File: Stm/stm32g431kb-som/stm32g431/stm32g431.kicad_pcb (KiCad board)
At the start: 2 copper layers, 30 x 26.8 mm, 4 parts, among them J1 Conn_ARM_JTAG_SWD_10, U1 STM32G431KBTx, Y1 ECS-TXO-3225-250-TR

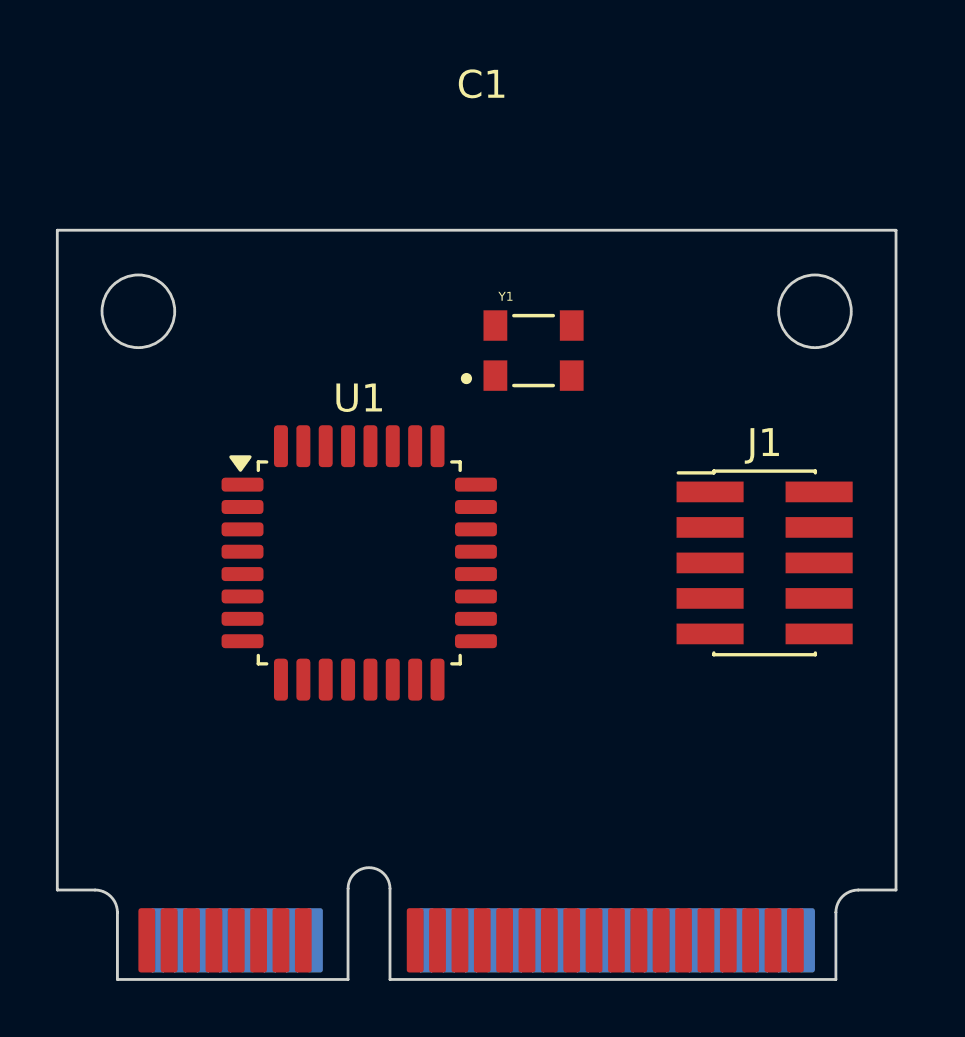
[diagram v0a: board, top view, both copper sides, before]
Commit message: Pcb
Add more components
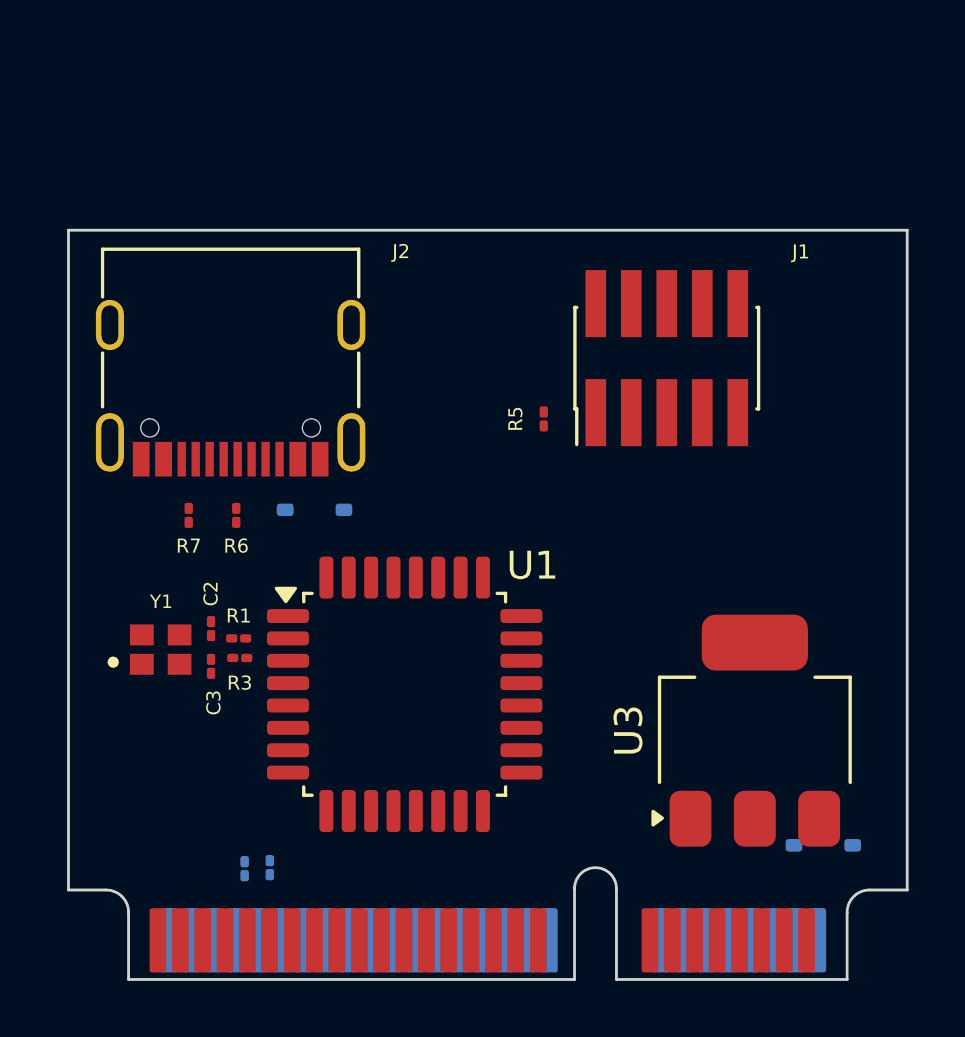
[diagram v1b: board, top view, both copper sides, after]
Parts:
- added C2: C, Capacitor_SMD:C_01005_0402Metric, F.Cu at (142.7, 87.8)
- added C3: C, Capacitor_SMD:C_01005_0402Metric, F.Cu at (142.7, 89.2)
- added D1: BAT60A, Diode_SMD:D_SOD-323, B.Cu at (146.4, 83.6)
- added D3: BAT60A, Diode_SMD:D_SOD-323, B.Cu at (164.6, 95.6)
- added J2: USB_C_Receptacle_USB2.0_16P, Connector_USB:USB_C_Receptacle_G-Switch_GT-USB-7010ASV, F.Cu at (143.4, 78.1)
- added R1: 0, Resistor_SMD:R_01005_0402Metric, F.Cu at (143.7, 88.2)
- added R2: 0, Resistor_SMD:R_01005_0402Metric, B.Cu at (143.9, 96.4)
- added R3: 0, Resistor_SMD:R_01005_0402Metric, F.Cu at (143.7, 88.9)
- added R4: 0, Resistor_SMD:R_01005_0402Metric, B.Cu at (144.8, 96.4)
- added R5: 0, Resistor_SMD:R_01005_0402Metric, F.Cu at (154.6, 80.3)
- added R6: 0, Resistor_SMD:R_01005_0402Metric, F.Cu at (143.6, 83.8)
- added R7: 0, Resistor_SMD:R_01005_0402Metric, F.Cu at (141.9, 83.8)
- added U3: LD1117S33TR_SOT223, Package_TO_SOT_SMD:SOT-223-3_TabPin2, F.Cu at (162.2, 91.5)
- C1: moved to B.Cu
- Y1: value ECS-TXO-3225-250-TR -> ECS-250-10-37B-CTN-TR; footprint User_Footprint:OSC_ECS-TXO-3225-250-TR -> User_Footprint:XTAL_ECS-160-9-37-CKM-TR
- moved Y1 17.1 mm to (140.9, 88.6)
- moved J1 8.12 mm to (159.0, 78.2), turned to 90 degrees
- moved U1 4.97 mm to (149.6, 90.2)
- turned C1 to 180 degrees
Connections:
- C1 pad 10: unconnected-(C1-Pad10) -> Net-(C1-Pad10)
- C1 pad 12: unconnected-(C1-Pad12) -> Net-(C1-Pad12)
- J1 pad 1: unconnected-(J1-VTref-Pad1) -> +3V3
- U1 pad 1: /VDD -> +3V3
- U1 pad 17: /VDD -> +3V3
- U1 pad 2: unconnected-(U1-PF0-Pad2) -> /PF0
- U1 pad 3: unconnected-(U1-PF1-Pad3) -> /PF1
- Y1 pad 1: unconnected-(Y1-VCONT-Pad1) -> /OSC_OUT
- Y1 pad 2: unconnected-(Y1-GND-Pad2) -> GND
- Y1 pad 3: unconnected-(Y1-OUTPUT-Pad3) -> /OSC_IN
- Y1 pad 4: +3.3V -> GND
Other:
- outline, holes or cut-outs redrawn

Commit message: SOM
Added Card Holes, Needed?
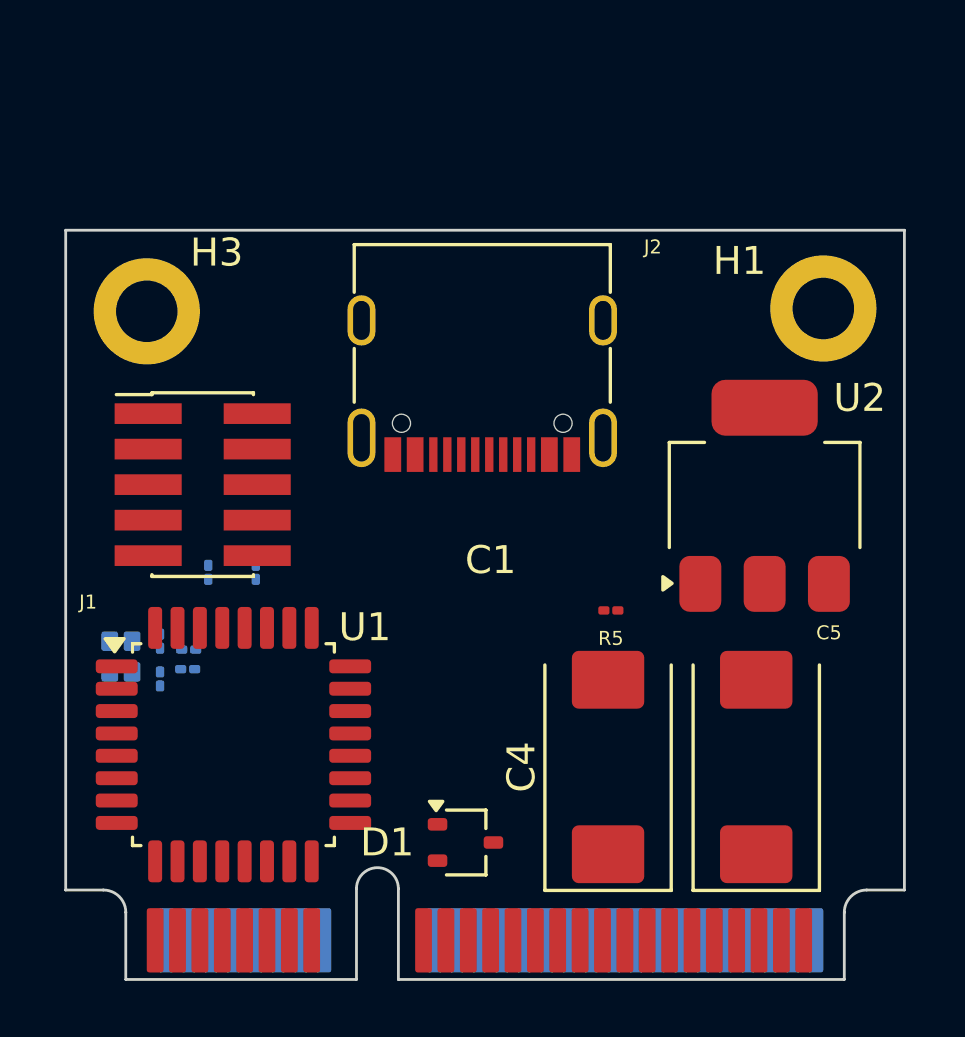
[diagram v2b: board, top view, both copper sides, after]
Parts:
- removed D3: BAT60A, Diode_SMD:D_SOD-323
- removed U3: LD1117S33TR_SOT223, Package_TO_SOT_SMD:SOT-223-3_TabPin2
- removed Y1: ECS-250-10-37B-CTN-TR, User_Footprint:XTAL_ECS-160-9-37-CKM-TR
- added C4: 22uF, Capacitor_Tantalum_SMD:CP_EIA-7343-30_AVX-N, F.Cu at (156.9, 92.8)
- added C5: 15uF, Capacitor_Tantalum_SMD:CP_EIA-7343-30_AVX-N, F.Cu at (162.2, 92.8)
- added H1: MountingHole_Pad, MountingHole:MountingHole_2.2mm_M2_DIN965_Pad, F.Cu at (164.6, 76.4)
- added H3: MountingHole_Pad, MountingHole:MountingHole_2.2mm_M2_DIN965_Pad, F.Cu at (140.4, 76.5)
- added U2: AP7361C-33E, Package_TO_SOT_SMD:SOT-223-3_TabPin2, F.Cu at (162.5, 83.1)
- added Y2: 24Mhz, User_Footprint:jxs11, B.Cu at (139.5, 88.9)
- C1: moved to F.Cu
- C2, C3, R1, R3, R6, R7: moved to B.Cu
- D1: value BAT60A -> BAT54CW; footprint Diode_SMD:D_SOD-323 -> Package_TO_SOT_SMD:SOT-323_SC-70; moved to F.Cu
- moved J1 17.2 mm to (142.4, 82.7), turned to 0 degrees
- moved D1 13.1 mm to (151.8, 95.5), turned to 0 degrees
- moved J2 9.00 mm to (152.4, 77.9)
- moved R5 7.26 mm to (157.0, 87.2), turned to 180 degrees
- moved U1 6.38 mm to (143.5, 92.0)
- moved C2 2.56 mm to (140.9, 89.7), turned to -90 degrees
- moved R6 2.15 mm to (144.3, 85.8), turned to 90 degrees
- moved R7 2.15 mm to (142.6, 85.8), turned to 90 degrees
- moved R1 2.13 mm to (141.9, 89.3)
- moved C3 2.03 mm to (140.9, 88.3), turned to 90 degrees
- moved R3 1.85 mm to (141.9, 88.6)
- moved C1 0.30 mm to (152.7, 85.4), turned to 0 degrees
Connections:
- C1 pad 9: unconnected-(C1-Pad9) -> /PG10
- D1 pad 1: Net-(D1-K) -> Net-(D1-Pad1)
- D1 pad 2: Net-(D1-A) -> /VDD
- J2 pad A4: Net-(D1-A) -> Net-(D1-Pad1)
- J2 pad A9: Net-(D1-A) -> Net-(D1-Pad1)
- J2 pad B4: Net-(D1-A) -> Net-(D1-Pad1)
- J2 pad B9: Net-(D1-A) -> Net-(D1-Pad1)
- U1 pad 15: unconnected-(U1-VDDA-Pad15) -> /VDDA
- U1 pad 4: unconnected-(U1-PG10-Pad4) -> /PG10
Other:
- outline, holes or cut-outs redrawn

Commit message: Pcb
Pre-final PCB
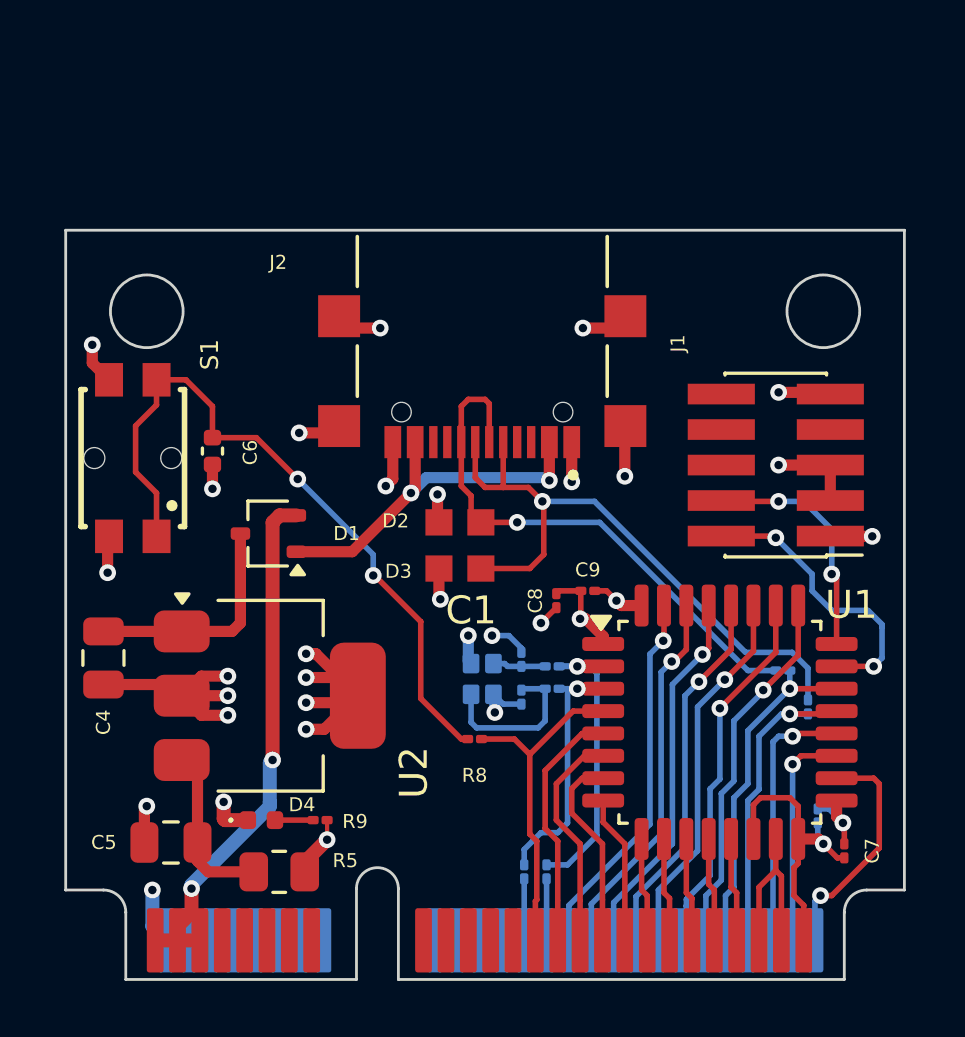
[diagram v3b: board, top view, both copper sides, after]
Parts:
- removed H1, H3: MountingHole_Pad, MountingHole:MountingHole_2.2mm_M2_DIN965_Pad
- added C10: 1uF, Capacitor_SMD:C_01005_0402Metric, B.Cu at (164.4, 94.5)
- added C6: 100nF, Capacitor_SMD:C_0402_1005Metric, F.Cu at (142.8, 81.5)
- added C7: 100nF, Capacitor_SMD:C_01005_0402Metric, F.Cu at (165.3, 95.8)
- added C8: 100nF, Capacitor_SMD:C_01005_0402Metric, F.Cu at (155.1, 86.8)
- added C9: 1uF, Capacitor_SMD:C_01005_0402Metric, F.Cu at (156.2, 86.5)
- added D2: PGB1010603NR, User_Footprint:DIOC1608X36N, F.Cu at (151.6, 84.0)
- added D3: PGB1010603NR, User_Footprint:DIOC1608X36N, F.Cu at (151.6, 85.7)
- added D4: LED, LED_SMD:LED_0402_1005Metric, F.Cu at (144.5, 94.7)
- added R8: 0, Resistor_SMD:R_01005_0402Metric, F.Cu at (152.1, 91.8)
- added R9: 100, Resistor_SMD:R_01005_0402Metric, F.Cu at (146.6, 94.7)
- added S1: 436331045822, User_Footprint:4363X10458XX, F.Cu at (139.9, 81.8)
- C4: value 22uF -> 1uF; footprint Capacitor_Tantalum_SMD:CP_EIA-7343-30_AVX-N -> Capacitor_SMD:C_0805_2012Metric
- C5: value 15uF -> 4.7uF; footprint Capacitor_Tantalum_SMD:CP_EIA-7343-30_AVX-N -> Capacitor_SMD:C_0805_2012Metric
- J2: footprint Connector_USB:USB_C_Receptacle_G-Switch_GT-USB-7010ASV -> User_Footprint:AMPHENOL_GSB1C41110SSHR
- R5: footprint Resistor_SMD:R_01005_0402Metric -> Resistor_SMD:R_0805_2012Metric
- moved C5 21.1 mm to (141.3, 95.5), turned to 180 degrees
- moved R7 20.8 mm to (163.2, 89.3), turned to 0 degrees
- moved J1 20.5 mm to (162.9, 82.0), turned to 180 degrees
- moved R6 20.3 mm to (164.1, 90.7), turned to -90 degrees
- moved U2 19.1 mm to (144.8, 90.2), turned to 0 degrees
- moved C4 18.5 mm to (138.8, 88.9), turned to -90 degrees
- moved U1 17.4 mm to (160.9, 91.2)
- moved R5 15.1 mm to (145.1, 96.5), turned to 0 degrees
- moved D1 13.1 mm to (144.8, 84.5), turned to 180 degrees
- moved C3 13.1 mm to (153.8, 90.3), turned to -90 degrees
- moved R3 13.1 mm to (154.9, 90.0)
- moved R1 13.0 mm to (154.9, 89.2)
- moved C2 12.9 mm to (153.8, 89.0), turned to 90 degrees
- moved Y2 12.9 mm to (152.4, 89.6), turned to 90 degrees
- moved R2 10.8 mm to (154.7, 96.5)
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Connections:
- C1 pad 10: Net-(C1-Pad10) -> unconnected-(C1-Pad10)
- C1 pad 12: Net-(C1-Pad12) -> unconnected-(C1-Pad12)
- C1 pad 13: /PA0 -> unconnected-(C1-Pad13)
- C1 pad 14: /PB0 -> unconnected-(C1-Pad14)
- C1 pad 15: /PA1 -> unconnected-(C1-Pad15)
- C1 pad 16: /PB3 -> unconnected-(C1-Pad16)
- C1 pad 17: /PA2 -> unconnected-(C1-Pad17)
- C1 pad 18: /PB4 -> unconnected-(C1-Pad18)
- C1 pad 19: /PA3 -> unconnected-(C1-Pad19)
- C1 pad 20: /PB5 -> unconnected-(C1-Pad20)
- C1 pad 21: /PA4 -> unconnected-(C1-Pad21)
- C1 pad 22: /PB6 -> unconnected-(C1-Pad22)
- C1 pad 23: /PA5 -> unconnected-(C1-Pad23)
- C1 pad 24: /PB7 -> unconnected-(C1-Pad24)
- C1 pad 25: /PA6 -> unconnected-(C1-Pad25)
- C1 pad 26: /PB8 -> /PFR1
- C1 pad 27: /PA7 -> /PG10
- C1 pad 28: unconnected-(C1-Pad28) -> /PFR0
- C1 pad 29: /PA8 -> /PA0
- C1 pad 30: unconnected-(C1-Pad30) -> /PB8
- C1 pad 31: /PA9 -> /PA1
- C1 pad 32: unconnected-(C1-Pad32) -> /PB7
- C1 pad 33: /PA10 -> /PA2
- C1 pad 34: unconnected-(C1-Pad34) -> /PB6
- C1 pad 35: /PA11 -> /PA3
- C1 pad 36: unconnected-(C1-Pad36) -> /PB5
- C1 pad 37: /PA12 -> /PA4
- C1 pad 38: unconnected-(C1-Pad38) -> /PB4
- C1 pad 39: /PA13 -> /PA5
- C1 pad 40: unconnected-(C1-Pad40) -> /PB3
- C1 pad 41: /PA14 -> /PA6
- C1 pad 42: unconnected-(C1-Pad42) -> /PA15
- C1 pad 43: /PA15 -> /PA7
- C1 pad 44: unconnected-(C1-Pad44) -> /PA12
- C1 pad 45: unconnected-(C1-Pad45) -> /PB0
- C1 pad 46: unconnected-(C1-Pad46) -> /PA11
- C1 pad 47: unconnected-(C1-Pad47) -> /VDDA
- C1 pad 48: unconnected-(C1-Pad48) -> /PA10
- C1 pad 49: unconnected-(C1-Pad49) -> /VDDA
- C1 pad 50: unconnected-(C1-Pad50) -> /PA9
- C1 pad 51: unconnected-(C1-Pad51) -> GND
- C1 pad 52: unconnected-(C1-Pad52) -> /PA8
- C1 pad 7: /VDDA -> unconnected-(C1-Pad7)
- C1 pad 9: /PG10 -> unconnected-(C1-Pad9)
- C4 pad 1: Net-(U2-VO) -> Net-(U2-VI)
- C5 pad 1: Net-(U2-VI) -> Net-(U2-VO)
- D1 pad 1: Net-(D1-Pad1) -> /VBUS
- R2 pad 1: Net-(C1-Pad10) -> /PFR0
- R4 pad 1: Net-(C1-Pad12) -> /PF1
- R4 pad 2: /PF1 -> /PFR1
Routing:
- net GND: track 0.00 -> 61.3 mm, vias 0 -> 29
- net Net-(C6-Pad1): track 0.00 -> 25.4 mm, vias 0 -> 2
- net /DM: track 0.00 -> 22.3 mm, vias 0 -> 1
- net /DP: track 0.00 -> 21.2 mm, vias 0 -> 1
- net /VDD: track 0.00 -> 18.9 mm, vias 0 -> 2
- net /PA15: track 0.00 -> 13.7 mm, vias 0 -> 1
- net /PB7: track 0.00 -> 13.4 mm, vias 0 -> 1
- net /PB8: track 0.00 -> 13.4 mm, vias 0 -> 1
- net /PB5: track 0.00 -> 13.4 mm, vias 0 -> 1
- net /PB4: track 0.00 -> 13.4 mm, vias 0 -> 1
- net /PB3: track 0.00 -> 13.4 mm, vias 0 -> 1
- net /PB6: track 0.00 -> 13.4 mm, vias 0 -> 1
- net /PA12: track 0.00 -> 12.6 mm, vias 0 -> 1
- net /VBUS: track 0.00 -> 12.4 mm, vias 0 -> 2
- net /PG10: track 0.00 -> 12.0 mm
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- added copper zone on In2.Cu, net +3V3
- added copper zone on In1.Cu, net GND
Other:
- outline, holes or cut-outs redrawn
- copper layers 2 -> 4
